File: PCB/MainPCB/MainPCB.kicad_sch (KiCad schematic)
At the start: 4 parts, among them J1 Conn_01x08_Socket, J2 Conn_01x06_Socket, U1 XB24CDMPIT-001, U2 DEV-16771

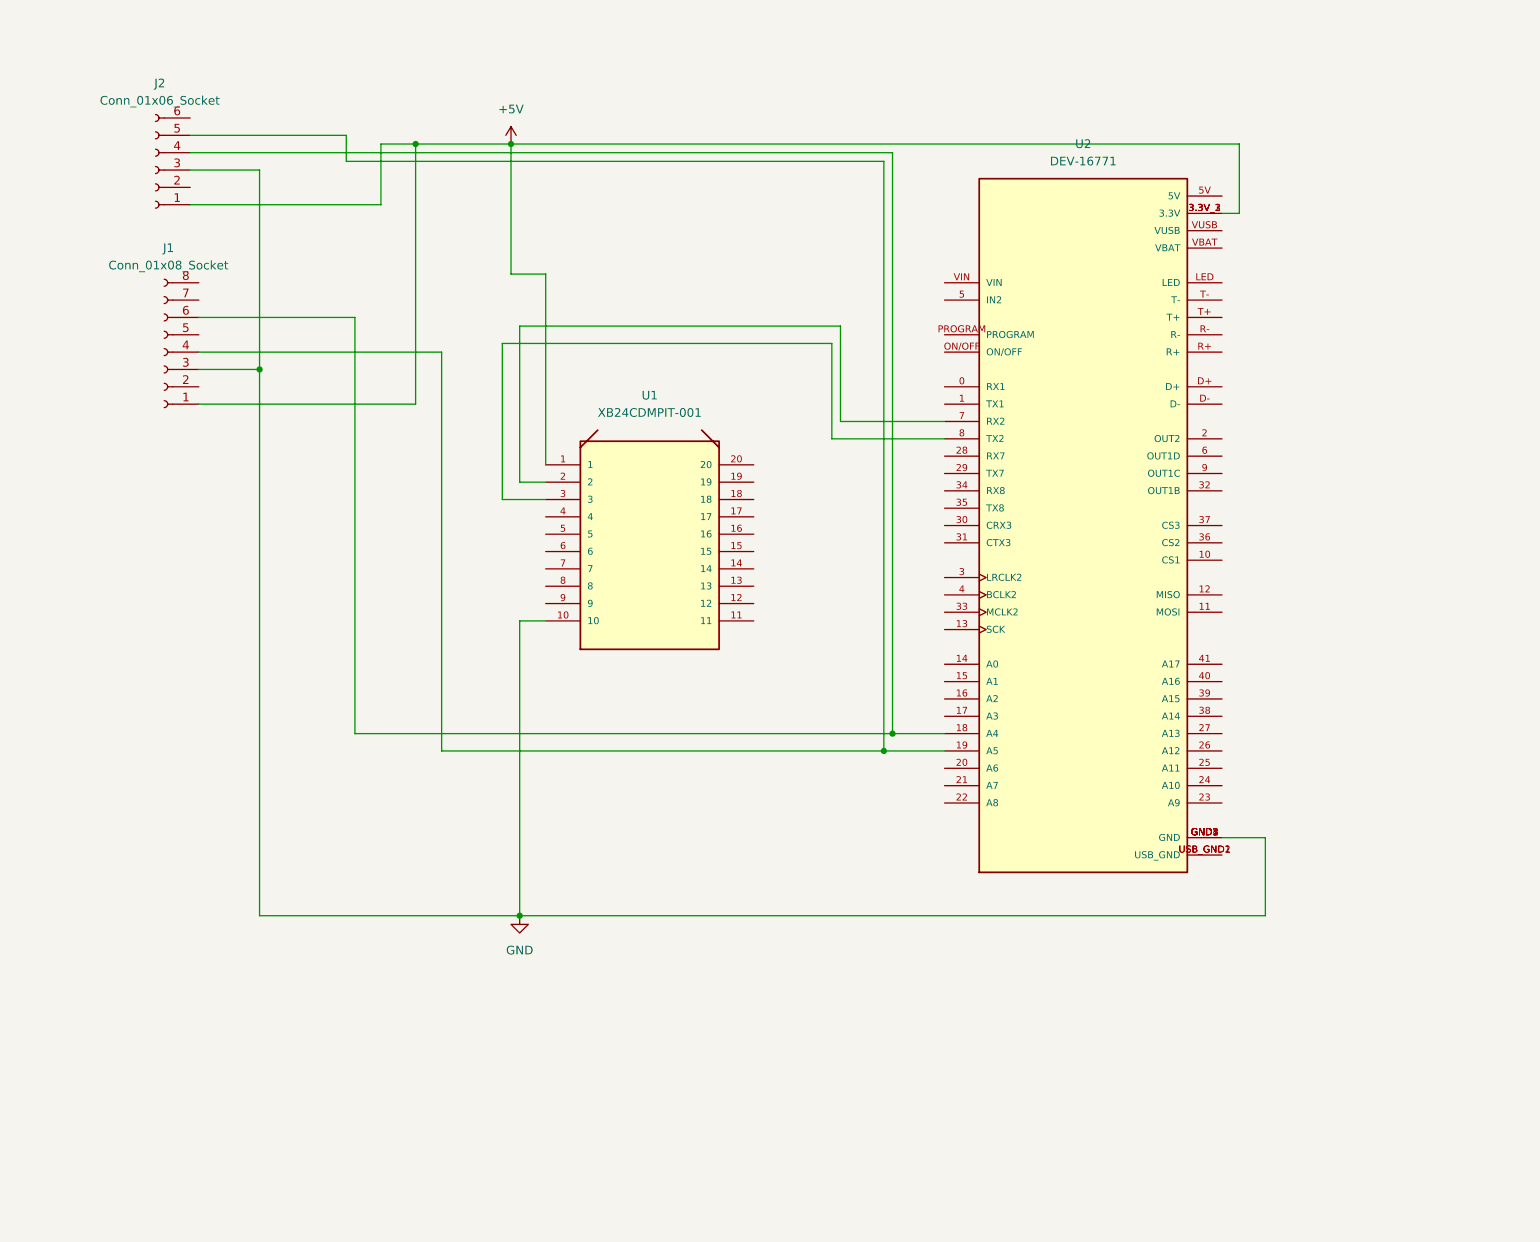
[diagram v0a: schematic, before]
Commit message: PCB.  'Tis done.
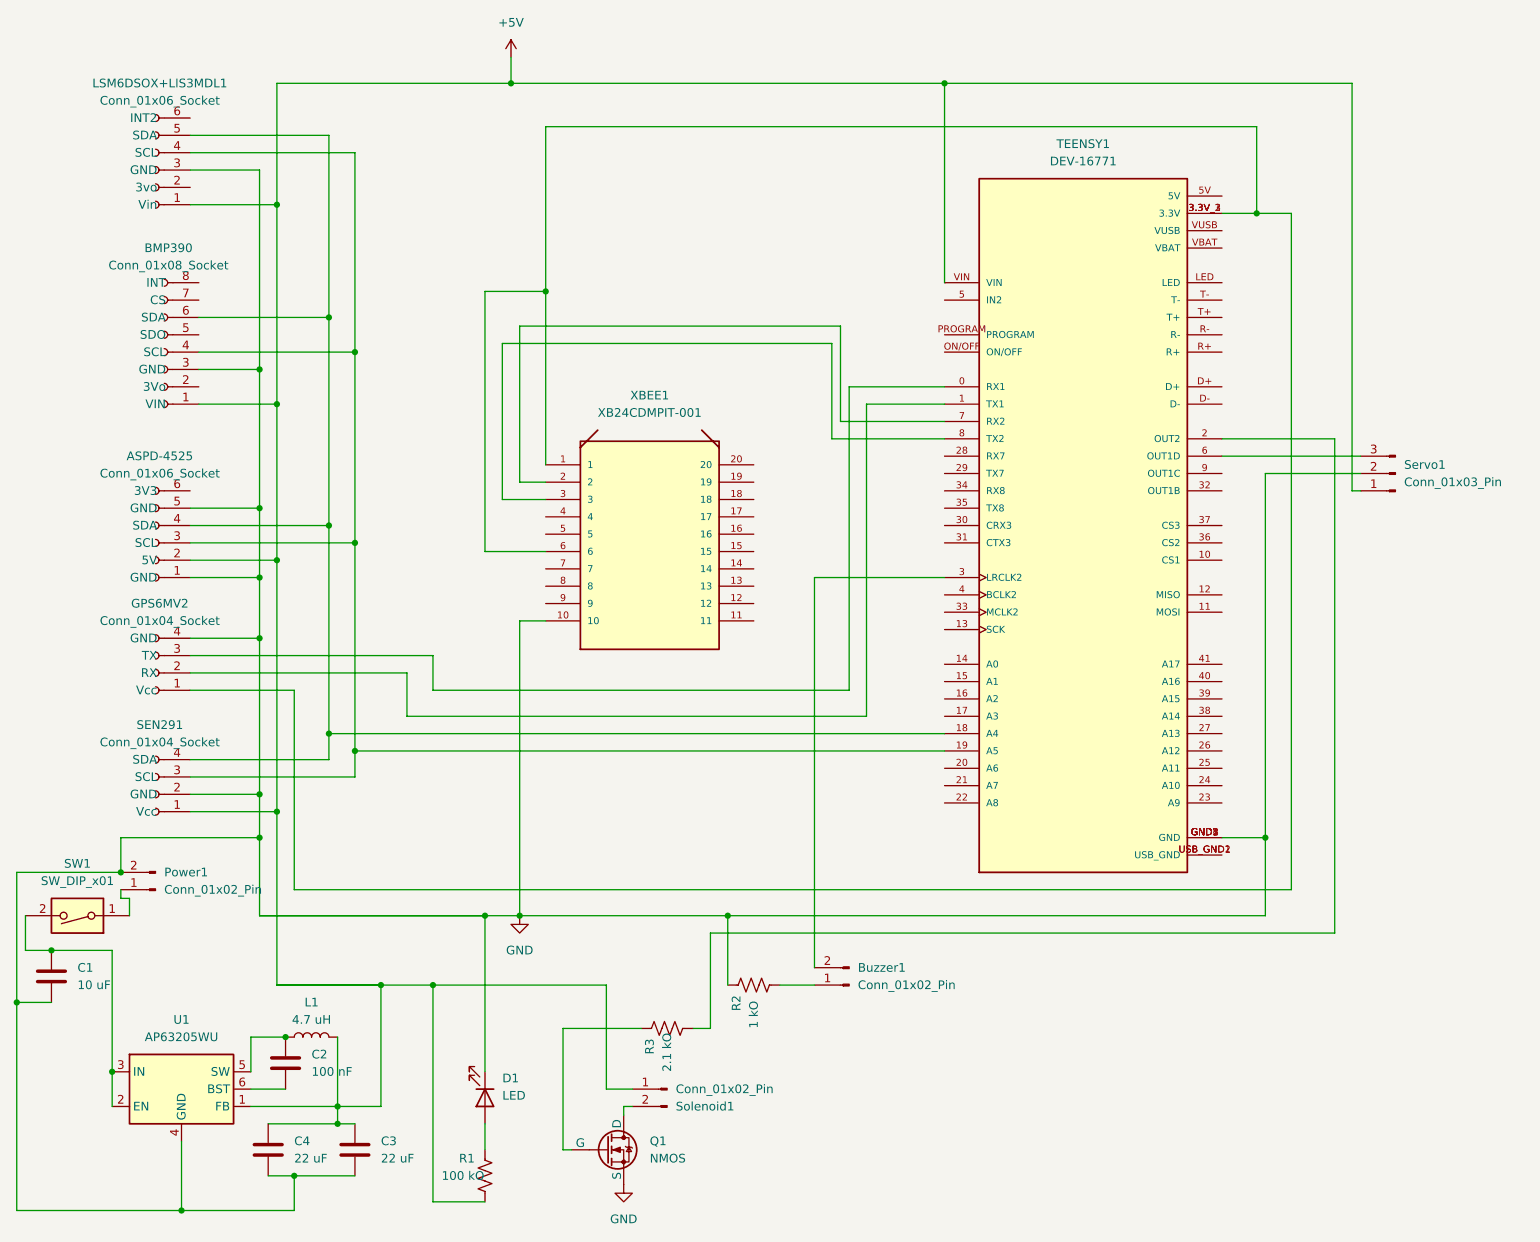
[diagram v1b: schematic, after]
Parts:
- added ASPD-4525: Conn_01x06_Socket, Connector_PinSocket_2.54mm:PinSocket_1x06_P2.54mm_Vertical, symbol Connector:Conn_01x06_Socket
- added Buzzer1: Conn_01x02_Pin, Connector_PinHeader_2.54mm:PinHeader_1x02_P2.54mm_Vertical, symbol Connector:Conn_01x02_Pin
- added C1: 10 uF, Capacitor_SMD:C_1206_3216Metric_Pad1.33x1.80mm_HandSolder, symbol Device:C
- added C2: 100 nF, Capacitor_SMD:C_0402_1005Metric_Pad0.74x0.62mm_HandSolder, symbol Device:C
- added C3, C4: 22 uF, Capacitor_SMD:C_0603_1608Metric_Pad1.08x0.95mm_HandSolder, symbol Device:C
- added D1: LED, Connector_PinSocket_2.54mm:PinSocket_1x02_P2.54mm_Vertical, symbol Device:LED
- added GPS6MV2, SEN291: Conn_01x04_Socket, Connector_PinSocket_2.54mm:PinSocket_1x04_P2.54mm_Vertical, symbol Connector:Conn_01x04_Socket
- added L1: 4.7 uH, Inductor_SMD:L_1008_2520Metric_Pad1.43x2.20mm_HandSolder, symbol Device:L
- added Power1, Solenoid1: Conn_01x02_Pin, Connector_PinSocket_2.54mm:PinSocket_1x02_P2.54mm_Vertical, symbol Connector:Conn_01x02_Pin
- added Q1: NMOS, Package_TO_SOT_THT:TO-220-3_Vertical, symbol Simulation_SPICE:NMOS
- added R1: 100 kO, Resistor_SMD:R_0402_1005Metric_Pad0.72x0.64mm_HandSolder, symbol Device:R_US
- added R2: 1 kO, Resistor_SMD:R_0402_1005Metric_Pad0.72x0.64mm_HandSolder, symbol Device:R_US
- added R3: 2.1 kO, Resistor_SMD:R_0603_1608Metric_Pad0.98x0.95mm_HandSolder, symbol Device:R_US
- added SW1: SW_DIP_x01, Connector_PinSocket_2.54mm:PinSocket_1x02_P2.54mm_Vertical, symbol Switch:SW_DIP_x01
- added Servo1: Conn_01x03_Pin, Connector_PinHeader_2.54mm:PinHeader_1x03_P2.54mm_Vertical, symbol Connector:Conn_01x03_Pin
- added U1: AP63205WU, Package_TO_SOT_SMD:TSOT-23-6, symbol Regulator_Switching:AP63205WU
- renumbered J1 to BMP390, J2 to LSM6DSOX+LIS3MDL1, U2 to TEENSY1, U1 to XBEE1
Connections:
- net +5V: now also TEENSY1.VIN, ASPD-4525.2 (5V), C3.2, C4.2, L1.2, R1.2, SEN291.1 (Vcc), Servo1.1 (Pin_1), Solenoid1.1 (Pin_1), U1.1 (FB); no longer TEENSY1.3.3V_1 (3.3V), TEENSY1.3.3V_2 (3.3V), TEENSY1.3.3V_3 (3.3V), XBEE1.1
- net GND: now also ASPD-4525.1 (GND), ASPD-4525.5 (GND), C1.2, C3.1, C4.1, D1.1 (K), GPS6MV2.4 (GND), Power1.2 (Pin_2), Q1.3 (S), R2.1, SEN291.2 (GND), Servo1.2 (Pin_2), U1.4 (GND)
- net at TEENSY1.0 (RX1): now also GPS6MV2.3 (TX)
- net at TEENSY1.1 (TX1): now also GPS6MV2.2 (RX)
- net at BMP390.6 (SDA), TEENSY1.18 (A4): now also LSM6DSOX+LIS3MDL1.5 (SDA), ASPD-4525.4 (SDA), SEN291.4 (SDA); no longer LSM6DSOX+LIS3MDL1.4 (Pin_4)
- net at BMP390.4 (SCL), TEENSY1.19 (A5): now also LSM6DSOX+LIS3MDL1.4 (SCL), ASPD-4525.3 (SCL), SEN291.3 (SCL); no longer LSM6DSOX+LIS3MDL1.5 (Pin_5)
- net at TEENSY1.2 (OUT2): now also R3.2
- net at TEENSY1.3 (LRCLK2): now also Buzzer1.2 (Pin_2)
- net at TEENSY1.6 (OUT1D): now also Servo1.3 (Pin_3)
- net at XBEE1.6: now also TEENSY1.3.3V_1 (3.3V), TEENSY1.3.3V_2 (3.3V), TEENSY1.3.3V_3 (3.3V), XBEE1.1, GPS6MV2.1 (Vcc)
- new net: Buzzer1.1 (Pin_1), R2.2
- new net: C1.1, SW1.2, U1.2 (EN), U1.3 (IN)
- new net: D1.2 (A), R1.1
- new net: C2.2, L1.1, U1.5 (SW)
- new net: Power1.1 (Pin_1), SW1.1
- new net: Q1.2 (G), R3.1
- new net: Q1.1 (D), Solenoid1.2 (Pin_2)
- new net: C2.1, U1.6 (BST)
